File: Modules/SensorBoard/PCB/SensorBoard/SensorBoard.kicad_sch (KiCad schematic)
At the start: 2 parts, among them J4 GPS

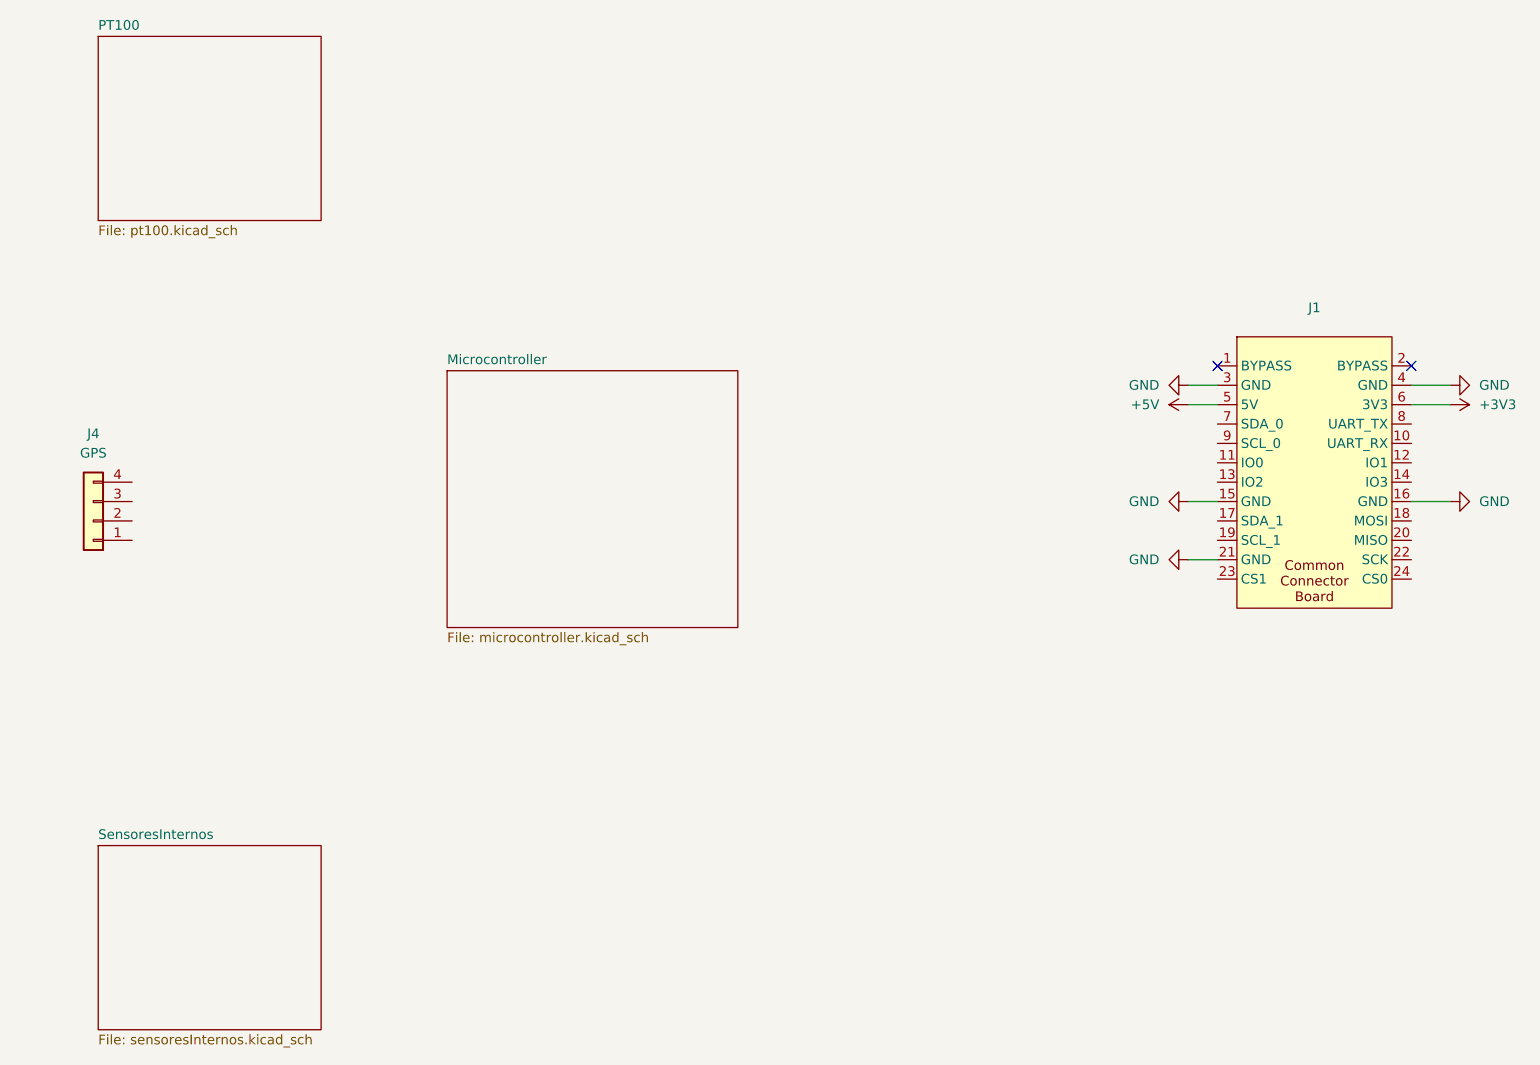
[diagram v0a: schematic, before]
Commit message: Finished Supply board
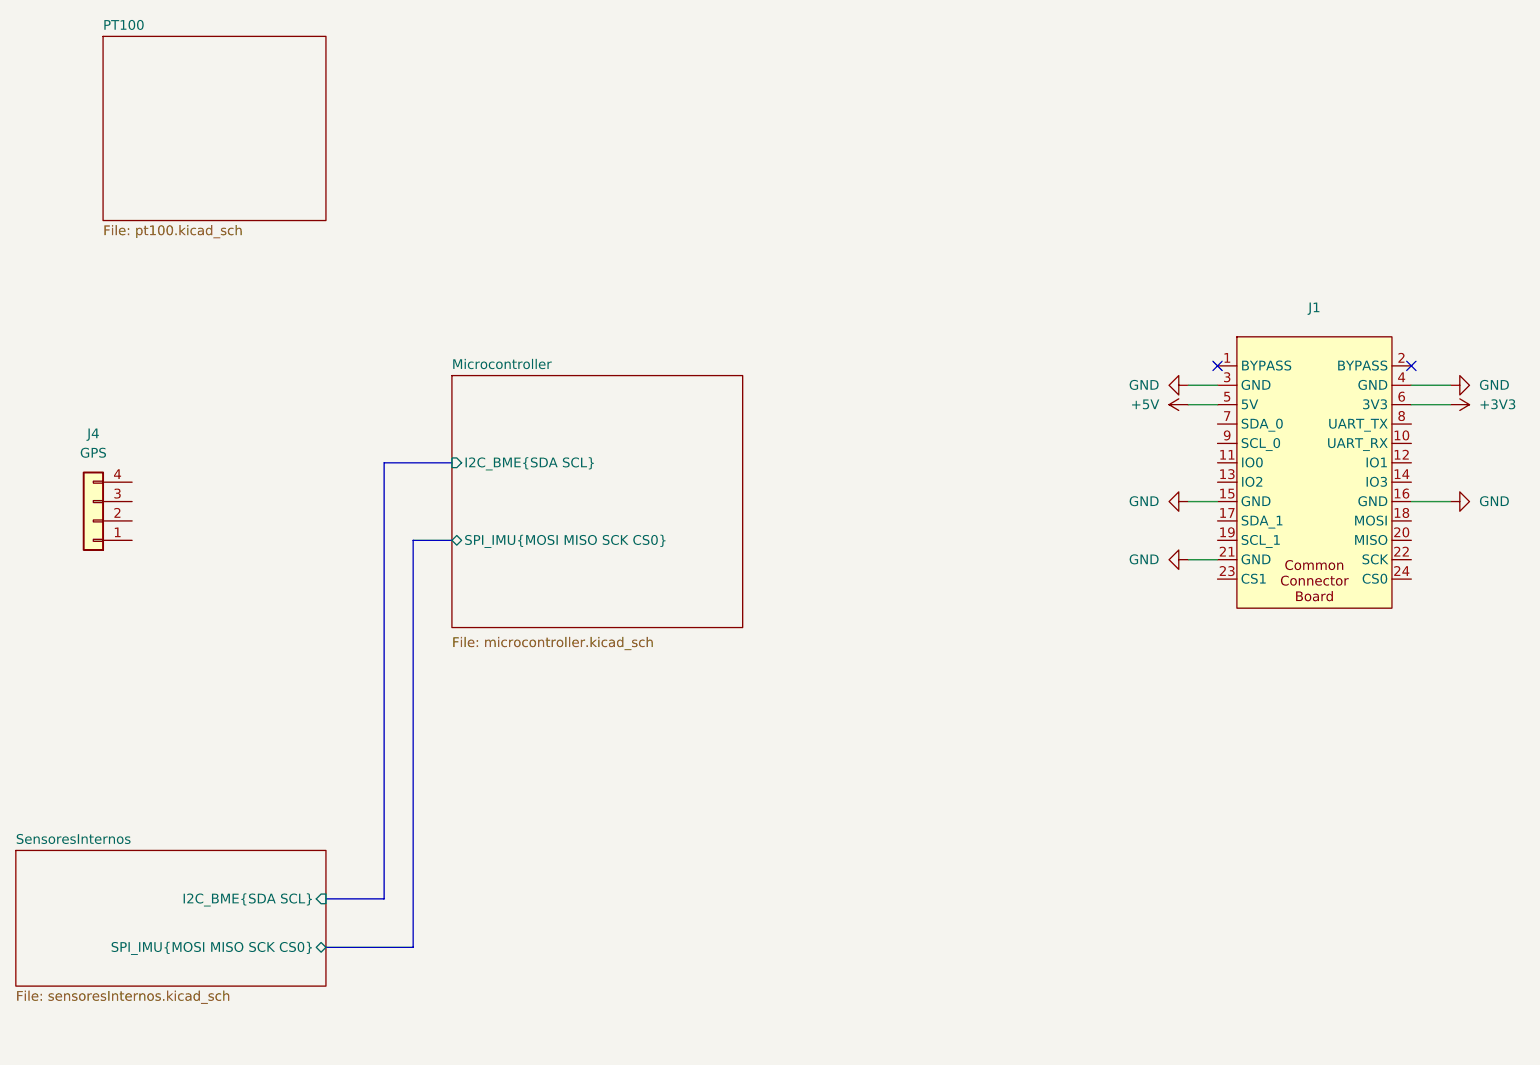
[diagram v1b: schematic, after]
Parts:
- J4: footprint Connector_JST:JST_PH_S4B-PH-K_1x04_P2.00mm_Horizontal -> Connector_JST:JST_ZH_S6B-ZR-SM4A-TF_1x06-1MP_P1.50mm_Horizontal
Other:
- sheet Microcontroller ports: added I2C_BME{SDA SCL}, SPI_IMU{MOSI MISO SCK CS0}; removed none
- sheet SensoresInternos ports: added I2C_BME{SDA SCL}, SPI_IMU{MOSI MISO SCK CS0}; removed none
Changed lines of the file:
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@@
 		(at 214.63 66.04)
 	)
+	(bus
+		(pts
+			(xy 105.41 135.89) (xy 105.41 78.74)
+		)
+		(stroke
+			(width 0)
+			(type default)
+		)
+	)
+	(bus
+		(pts
+			(xy 97.79 135.89) (xy 105.41 135.89)
+		)
+		(stroke
+			(width 0)
+			(type default)
+		)
+	)
 	(wire
 		(pts
@@
 		)
 	)
+	(bus
+		(pts
+			(xy 109.22 88.9) (xy 114.3 88.9)
+		)
+		(stroke
+			(width 0)
+			(type default)
+		)
+	)
 	(wire
 		(pts
@@
 		)
 	)
+	(bus
+		(pts
+			(xy 97.79 142.24) (xy 109.22 142.24)
+		)
+		(stroke
+			(width 0)
+			(type default)
+		)
+	)
 	(wire
 		(pts
@@
 		(pts
 			(xy 210.82 71.12) (xy 214.63 71.12)
+		)
+		(stroke
+			(width 0)
+			(type default)
+		)
+	)
+	(bus
+		(pts
+			(xy 109.22 142.24) (xy 109.22 88.9)
+		)
+		(stroke
+			(width 0)
+			(type default)
+		)
+	)
+	(bus
+		(pts
+			(xy 105.41 78.74) (xy 114.3 78.74)
 		)
 		(stroke
@@
 			)
 		)
-		(property "Footprint" "Connector_JST:JST_PH_S4B-PH-K_1x04_P2.00mm_Horizontal"
+		(property "Footprint" "Connector_JST:JST_ZH_S6B-ZR-SM4A-TF_1x06-1MP_P1.50mm_Horizontal"
 			(at 67.31 86.36 0)
 			(effects
@@
 	)
 	(sheet
-		(at 67.945 22.86)
+		(at 68.58 22.86)
 		(size 29.21 24.13)
 		(exclude_from_sim no)
@@
 		)
 		(property "Sheetname" "PT100"
-			(at 67.945 22.1484 0)
+			(at 68.58 22.1484 0)
 			(effects
 				(font
@@
 		)
 		(property "Sheetfile" "pt100.kicad_sch"
-			(at 67.945 47.5746 0)
+			(at 68.58 47.5746 0)
 			(effects
 				(font
@@
 	)
 	(sheet
-		(at 113.665 66.675)
-		(size 38.1 33.655)
+		(at 114.3 67.31)
+		(size 38.1 33.02)
 		(exclude_from_sim no)
 		(in_bom yes)
@@
 		)
 		(property "Sheetname" "Microcontroller"
-			(at 113.665 65.9634 0)
+			(at 114.3 66.5984 0)
 			(effects
 				(font
@@
 		)
 		(property "Sheetfile" "microcontroller.kicad_sch"
-			(at 113.665 100.9146 0)
+			(at 114.3 101.5496 0)
 			(effects
 				(font
@@
 			)
 		)
+		(pin "I2C_BME{SDA SCL}" input
+			(at 114.3 78.74 180)
+			(effects
+				(font
+					(size 1.27 1.27)
+				)
+				(justify left)
+			)
+		)
+		(pin "SPI_IMU{MOSI MISO SCK CS0}" bidirectional
+			(at 114.3 88.9 180)
+			(effects
+				(font
+					(size 1.27 1.27)
+				)
+				(justify left)
+			)
+		)
 		(instances
 			(project "SensorBoard"
@@
 	)
 	(sheet
-		(at 67.945 128.905)
-		(size 29.21 24.13)
+		(at 57.15 129.54)
+		(size 40.64 17.78)
 		(exclude_from_sim no)
 		(in_bom yes)
@@
 		)
 		(property "Sheetname" "SensoresInternos"
-			(at 67.945 128.1934 0)
+			(at 57.15 128.8284 0)
 			(effects
 				(font
@@
 		)
 		(property "Sheetfile" "sensoresInternos.kicad_sch"
-			(at 67.945 153.6196 0)
+			(at 57.15 147.9046 0)
 			(effects
 				(font
@@
 			)
 		)
+		(pin "I2C_BME{SDA SCL}" input
+			(at 97.79 135.89 0)
+			(effects
+				(font
+					(size 1.27 1.27)
+				)
+				(justify right)
+			)
+		)
+		(pin "SPI_IMU{MOSI MISO SCK CS0}" bidirectional
+			(at 97.79 142.24 0)
+			(effects
+				(font
+					(size 1.27 1.27)
+				)
+				(justify right)
+			)
+		)
